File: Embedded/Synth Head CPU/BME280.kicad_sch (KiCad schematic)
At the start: 3 parts, among them U2 BME280

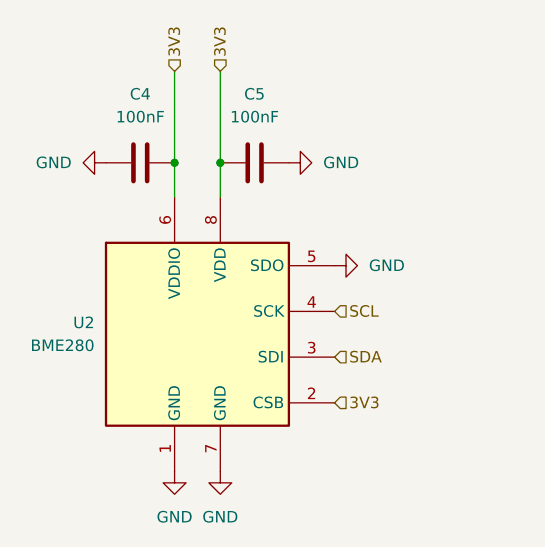
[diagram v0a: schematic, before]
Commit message: Prepared All Main Boards for PCB Creation
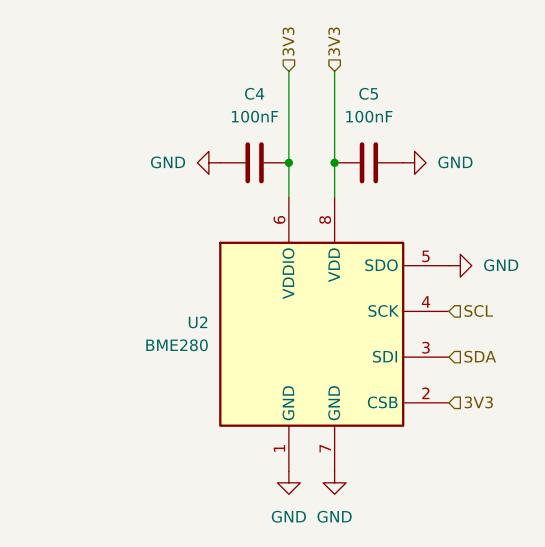
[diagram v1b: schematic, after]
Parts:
- C4, C5: footprint (none) -> Capacitor_SMD:C_0603_1608Metric_Pad1.08x0.95mm_HandSolder
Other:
- moved on the sheet: C4, C5, U2
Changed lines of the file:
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@@
 	(paper "A4")
 	(junction
-		(at 127 80.01)
+		(at 139.7 80.01)
 		(diameter 0)
 		(color 0 0 0 0)
 	)
 	(junction
-		(at 121.92 80.01)
+		(at 134.62 80.01)
 		(diameter 0)
 		(color 0 0 0 0)
@@
 	(wire
 		(pts
-			(xy 127 80.01) (xy 127 83.82)
+			(xy 139.7 80.01) (xy 139.7 83.82)
 		)
 		(stroke
@@
 	(wire
 		(pts
-			(xy 121.92 69.85) (xy 121.92 80.01)
+			(xy 134.62 69.85) (xy 134.62 80.01)
 		)
 		(stroke
@@
 	(wire
 		(pts
-			(xy 121.92 80.01) (xy 121.92 83.82)
+			(xy 134.62 80.01) (xy 134.62 83.82)
 		)
 		(stroke
@@
 	(wire
 		(pts
-			(xy 127 69.85) (xy 127 80.01)
+			(xy 139.7 69.85) (xy 139.7 80.01)
 		)
 		(stroke
@@
 	(hierarchical_label "SCL"
 		(shape input)
-		(at 139.7 96.52 0)
+		(at 152.4 96.52 0)
 		(fields_autoplaced yes)
 		(effects
@@
 	(hierarchical_label "3V3"
 		(shape input)
-		(at 139.7 106.68 0)
+		(at 152.4 106.68 0)
 		(fields_autoplaced yes)
 		(effects
@@
 	(hierarchical_label "3V3"
 		(shape input)
-		(at 121.92 69.85 90)
+		(at 134.62 69.85 90)
 		(fields_autoplaced yes)
 		(effects
@@
 	(hierarchical_label "SDA"
 		(shape input)
-		(at 139.7 101.6 0)
+		(at 152.4 101.6 0)
 		(fields_autoplaced yes)
 		(effects
@@
 	(hierarchical_label "3V3"
 		(shape input)
-		(at 127 69.85 90)
+		(at 139.7 69.85 90)
 		(fields_autoplaced yes)
 		(effects
@@
 	(symbol
 		(lib_id "Device:C")
-		(at 118.11 80.01 90)
+		(at 130.81 80.01 90)
 		(unit 1)
 		(exclude_from_sim no)
@@
 		(fields_autoplaced yes)
 		(property "Reference" "C4"
-			(at 118.11 72.39 90)
+			(at 130.81 72.39 90)
 			(effects
 				(font
@@
 		)
 		(property "Value" "100nF"
-			(at 118.11 74.93 90)
-			(effects
-				(font
-					(size 1.27 1.27)
-				)
-			)
-		)
-		(property "Footprint" ""
-			(at 121.92 79.0448 0)
+			(at 130.81 74.93 90)
+			(effects
+				(font
+					(size 1.27 1.27)
+				)
+			)
+		)
+		(property "Footprint" "Capacitor_SMD:C_0603_1608Metric_Pad1.08x0.95mm_HandSolder"
+			(at 134.62 79.0448 0)
 			(effects
 				(font
@@
 		)
 		(property "Datasheet" "~"
-			(at 118.11 80.01 0)
+			(at 130.81 80.01 0)
 			(effects
 				(font
@@
 		)
 		(property "Description" "Unpolarized capacitor"
-			(at 118.11 80.01 0)
+			(at 130.81 80.01 0)
 			(effects
 				(font
@@
 	(symbol
 		(lib_id "power:GND")
-		(at 134.62 80.01 90)
+		(at 147.32 80.01 90)
 		(unit 1)
 		(exclude_from_sim no)
@@
 		(fields_autoplaced yes)
 		(property "Reference" "#PWR012"
-			(at 140.97 80.01 0)
+			(at 153.67 80.01 0)
 			(effects
 				(font
@@
 		)
 		(property "Value" "GND"
-			(at 138.43 80.0099 90)
+			(at 151.13 80.0099 90)
 			(effects
 				(font
@@
 		)
 		(property "Footprint" ""
-			(at 134.62 80.01 0)
+			(at 147.32 80.01 0)
 			(effects
 				(font
@@
 		)
 		(property "Datasheet" ""
-			(at 134.62 80.01 0)
+			(at 147.32 80.01 0)
 			(effects
 				(font
@@
 		)
 		(property "Description" "Power symbol creates a global label with name \"GND\" , ground"
-			(at 134.62 80.01 0)
+			(at 147.32 80.01 0)
 			(effects
 				(font
@@
 	(symbol
 		(lib_id "Sensor:BME280")
-		(at 124.46 99.06 0)
+		(at 137.16 99.06 0)
 		(unit 1)
 		(exclude_from_sim no)
@@
 		(fields_autoplaced yes)
 		(property "Reference" "U2"
-			(at 113.03 97.7899 0)
+			(at 125.73 97.7899 0)
 			(effects
 				(font
@@
 		)
 		(property "Value" "BME280"
-			(at 113.03 100.3299 0)
+			(at 125.73 100.3299 0)
 			(effects
 				(font
@@
 		)
 		(property "Footprint" "Package_LGA:Bosch_LGA-8_2.5x2.5mm_P0.65mm_ClockwisePinNumbering"
-			(at 162.56 110.49 0)
+			(at 175.26 110.49 0)
 			(effects
 				(font
@@
 		)
 		(property "Datasheet" "https://www.bosch-sensortec.com/media/boschsensortec/downloads/datasheets/bst-bme280-ds002.pdf"
-			(at 124.46 104.14 0)
+			(at 137.16 104.14 0)
 			(effects
 				(font
@@
 		)
 		(property "Description" "3-in-1 sensor, humidity, pressure, temperature, I2C and SPI interface, 1.71-3.6V, LGA-8"
-			(at 124.46 99.06 0)
+			(at 137.16 99.06 0)
 			(effects
 				(font
@@
 	(symbol
 		(lib_id "power:GND")
-		(at 121.92 114.3 0)
+		(at 134.62 114.3 0)
 		(unit 1)
 		(exclude_from_sim no)
@@
 		(fields_autoplaced yes)
 		(property "Reference" "#PWR010"
-			(at 121.92 120.65 0)
+			(at 134.62 120.65 0)
 			(effects
 				(font
@@
 		)
 		(property "Value" "GND"
-			(at 121.92 119.38 0)
+			(at 134.62 119.38 0)
 			(effects
 				(font
@@
 		)
 		(property "Footprint" ""
-			(at 121.92 114.3 0)
+			(at 134.62 114.3 0)
 			(effects
 				(font
@@
 		)
 		(property "Datasheet" ""
-			(at 121.92 114.3 0)
+			(at 134.62 114.3 0)
 			(effects
 				(font
@@
 		)
 		(property "Description" "Power symbol creates a global label with name \"GND\" , ground"
-			(at 121.92 114.3 0)
+			(at 134.62 114.3 0)
 			(effects
 				(font
@@
 	(symbol
 		(lib_id "power:GND")
-		(at 127 114.3 0)
+		(at 139.7 114.3 0)
 		(unit 1)
 		(exclude_from_sim no)
@@
 		(fields_autoplaced yes)
 		(property "Reference" "#PWR011"
-			(at 127 120.65 0)
+			(at 139.7 120.65 0)
 			(effects
 				(font
@@
 		)
 		(property "Value" "GND"
-			(at 127 119.38 0)
+			(at 139.7 119.38 0)
 			(effects
 				(font
@@
 		)
 		(property "Footprint" ""
-			(at 127 114.3 0)
+			(at 139.7 114.3 0)
 			(effects
 				(font
@@
 		)
 		(property "Datasheet" ""
-			(at 127 114.3 0)
+			(at 139.7 114.3 0)
 			(effects
 				(font
@@
 		)
 		(property "Description" "Power symbol creates a global label with name \"GND\" , ground"
-			(at 127 114.3 0)
+			(at 139.7 114.3 0)
 			(effects
 				(font
@@
 	(symbol
 		(lib_id "power:GND")
-		(at 139.7 91.44 90)
+		(at 152.4 91.44 90)
 		(unit 1)
 		(exclude_from_sim no)
@@
 		(fields_autoplaced yes)
 		(property "Reference" "#PWR013"
-			(at 146.05 91.44 0)
+			(at 158.75 91.44 0)
 			(effects
 				(font
@@
 		)
 		(property "Value" "GND"
-			(at 143.51 91.4399 90)
+			(at 156.21 91.4399 90)
 			(effects
 				(font
@@
 		)
 		(property "Footprint" ""
-			(at 139.7 91.44 0)
+			(at 152.4 91.44 0)
 			(effects
 				(font
@@
 		)
 		(property "Datasheet" ""
-			(at 139.7 91.44 0)
+			(at 152.4 91.44 0)
 			(effects
 				(font
@@
 		)
 		(property "Description" "Power symbol creates a global label with name \"GND\" , ground"
-			(at 139.7 91.44 0)
+			(at 152.4 91.44 0)
 			(effects
 				(font
@@
 	(symbol
 		(lib_id "Device:C")
-		(at 130.81 80.01 90)
+		(at 143.51 80.01 90)
 		(unit 1)
 		(exclude_from_sim no)
@@
 		(fields_autoplaced yes)
 		(property "Reference" "C5"
-			(at 130.81 72.39 90)
+			(at 143.51 72.39 90)
 			(effects
 				(font
@@
 		)
 		(property "Value" "100nF"
-			(at 130.81 74.93 90)
-			(effects
-				(font
-					(size 1.27 1.27)
-				)
-			)
-		)
-		(property "Footprint" ""
-			(at 134.62 79.0448 0)
+			(at 143.51 74.93 90)
+			(effects
+				(font
+					(size 1.27 1.27)
+				)
+			)
+		)
+		(property "Footprint" "Capacitor_SMD:C_0603_1608Metric_Pad1.08x0.95mm_HandSolder"
+			(at 147.32 79.0448 0)
 			(effects
 				(font
@@
 		)
 		(property "Datasheet" "~"
-			(at 130.81 80.01 0)
+			(at 143.51 80.01 0)
 			(effects
 				(font
@@
 		)
 		(property "Description" "Unpolarized capacitor"
-			(at 130.81 80.01 0)
+			(at 143.51 80.01 0)
 			(effects
 				(font
@@
 	(symbol
 		(lib_id "power:GND")
-		(at 114.3 80.01 270)
+		(at 127 80.01 270)
 		(unit 1)
 		(exclude_from_sim no)
@@
 		(fields_autoplaced yes)
 		(property "Reference" "#PWR09"
-			(at 107.95 80.01 0)
+			(at 120.65 80.01 0)
 			(effects
 				(font
@@
 		)
 		(property "Value" "GND"
-			(at 110.49 80.0099 90)
+			(at 123.19 80.0099 90)
 			(effects
 				(font
@@
 		)
 		(property "Footprint" ""
-			(at 114.3 80.01 0)
+			(at 127 80.01 0)
 			(effects
 				(font
@@
 		)
 		(property "Datasheet" ""
-			(at 114.3 80.01 0)
+			(at 127 80.01 0)
 			(effects
 				(font
@@
 		)
 		(property "Description" "Power symbol creates a global label with name \"GND\" , ground"
-			(at 114.3 80.01 0)
-			(effects
-				(font
+			(at 127 80.01 0)
+			(effects
+				(font
